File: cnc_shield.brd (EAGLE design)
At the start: 160 x 100 mm, 17 parts, among them X4 1751248

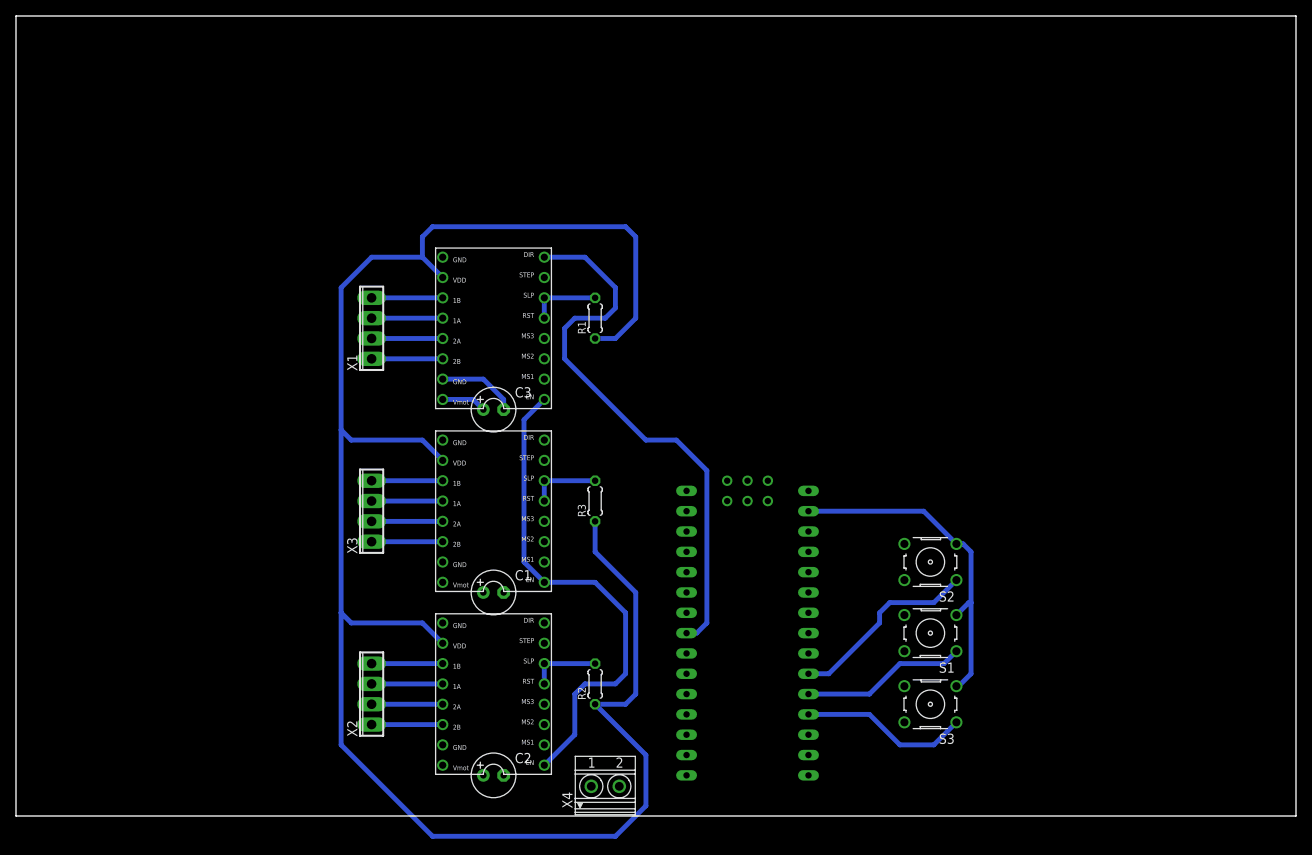
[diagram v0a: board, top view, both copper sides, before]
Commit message: primeira versao completa da board
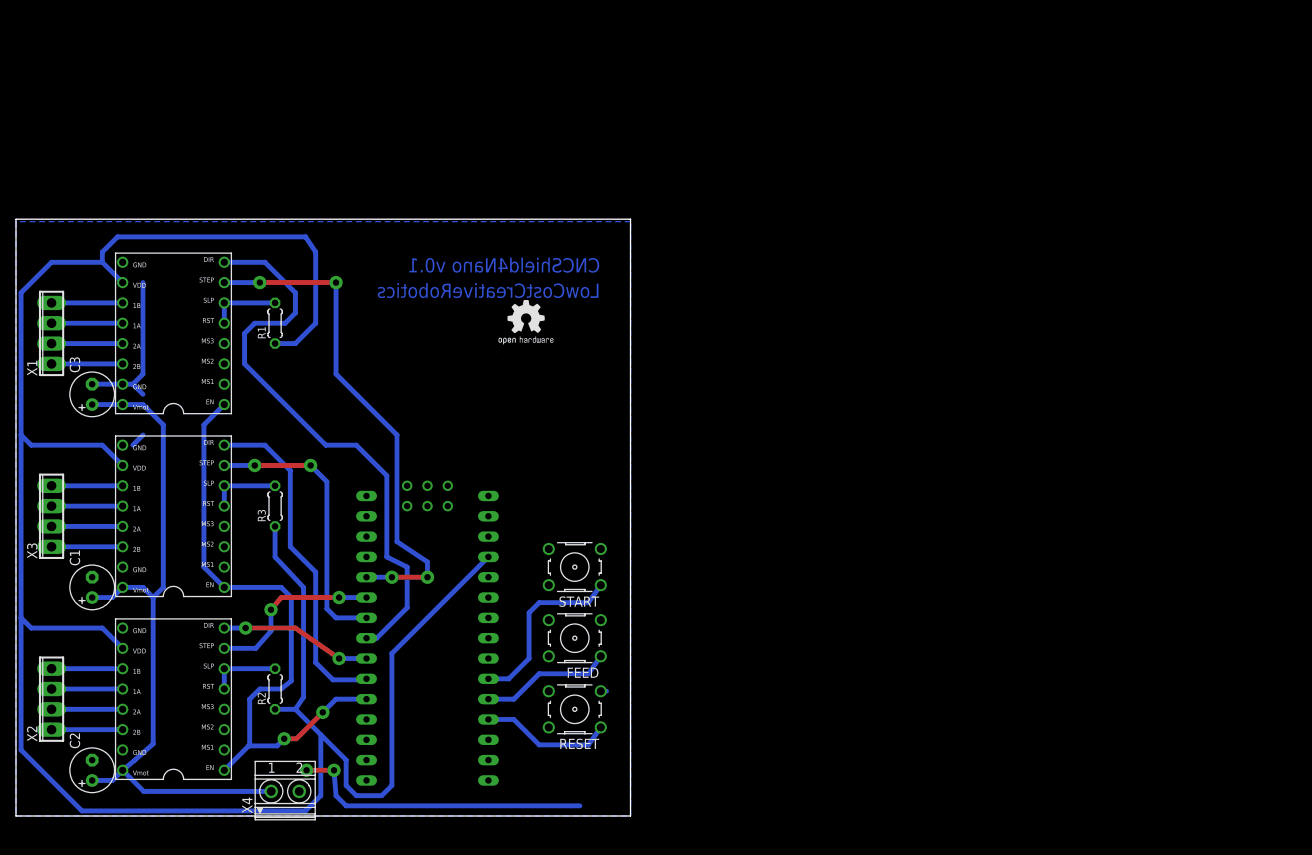
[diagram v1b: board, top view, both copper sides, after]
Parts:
- removed S1, S2, S3: (no value), RepRapjr:B3F-10XX-RPAD
- added FEED, RESET, START: (no value), RepRapjr:B3F-10XX-RPAD
- added GOLD_ORB_SM1: OSHWLOGO_GOLD_ORB_SM, NBitWonder:OSHW2
- C1, C2, C3: value (none) -> 10UF/30V
- X1: value (none) -> MOTOR 1
- X2: value (none) -> MOTOR 2
- X3: value (none) -> MOTOR 3
- moved C3 50.2 mm to (9.53, 52.7), turned to 90 degrees
- moved C1 50.2 mm to (9.53, 28.6), turned to 90 degrees
- moved C2 50.2 mm to (9.53, 5.71), turned to 90 degrees
- moved R1 40.0 mm to (32.4, 61.6)
- moved R2 40.0 mm to (32.4, 15.9)
- moved R3 40.0 mm to (32.4, 38.7)
- moved U$1 40.0 mm to (48.9, 31.1)
- moved X1 40.0 mm to (4.45, 60.3)
- moved X2 40.0 mm to (4.45, 14.6)
- moved X3 40.0 mm to (4.45, 37.5)
- moved U$2 40.0 mm to (14.6, 6.99)
- moved U$3 40.0 mm to (14.6, 29.8)
- moved U$4 40.0 mm to (14.6, 52.7)
- moved X4 40.0 mm to (33.7, 3.17)
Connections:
- removed net N$22: U$1.D8
- net ENABLE: now also U$1.D8
- net GND: now also FEED.3, RESET.3, START.3; no longer S1.3, S2.3, S3.3
- net N$16: now also RESET.1; no longer S3.1
- net N$17: now also FEED.1; no longer S1.1
- net N$18: now also START.1; no longer S2.1
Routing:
- net V_MOT: track 5.61 -> 88.1 mm
- net STEP_M1: track 0.00 -> 63.6 mm, vias 0 -> 4
- net DIR_M3: track 0.00 -> 42.2 mm
- net VCC: track 236.6 -> 274.4 mm
- net STEP_M3: track 0.00 -> 35.0 mm, vias 0 -> 2
- net STEP_M2: track 0.00 -> 22.1 mm, vias 0 -> 2
- net DIR_M2: track 0.00 -> 19.0 mm, vias 0 -> 2
- net ENABLE: track 62.2 -> 77.7 mm, vias 0 -> 2
- net GND: track 52.5 -> 60.7 mm, vias 0 -> 2
- net N$16: track 21.2 -> 16.5 mm
- net N$17: track 20.7 -> 16.5 mm
- net DIR_M1: track 69.9 -> 72.5 mm
- net N$18: track 24.1 -> 22.5 mm
- added copper zone on layer 16, net GND
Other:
- board size 160 x 100 mm -> 76.8 x 74.6 mm
- board text added: "CNCShield4Nano"
- board text added: "CNCShield4Nano v0.1"
- board text added: "LowCostCreativeRobotics"
